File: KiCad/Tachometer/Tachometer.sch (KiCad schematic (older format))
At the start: 24 parts, among them J1 PJ301M-12, Q1 2N3904, Q2 2N3904

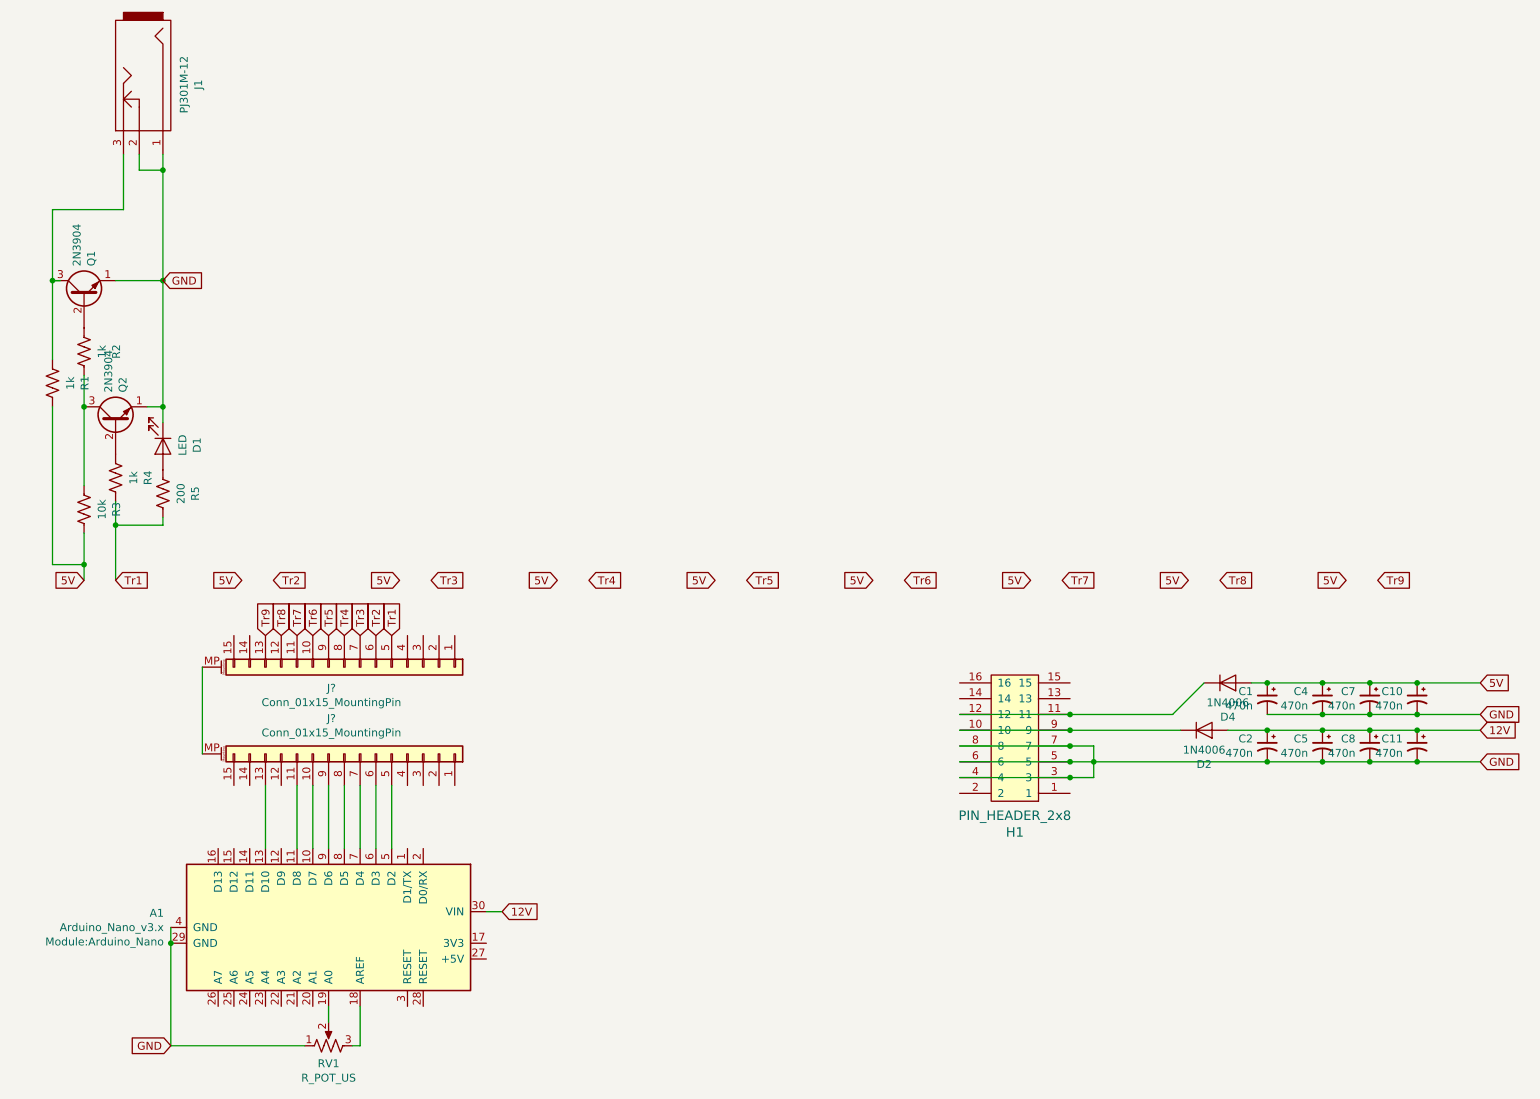
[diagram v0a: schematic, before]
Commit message: ruffplaced pcb
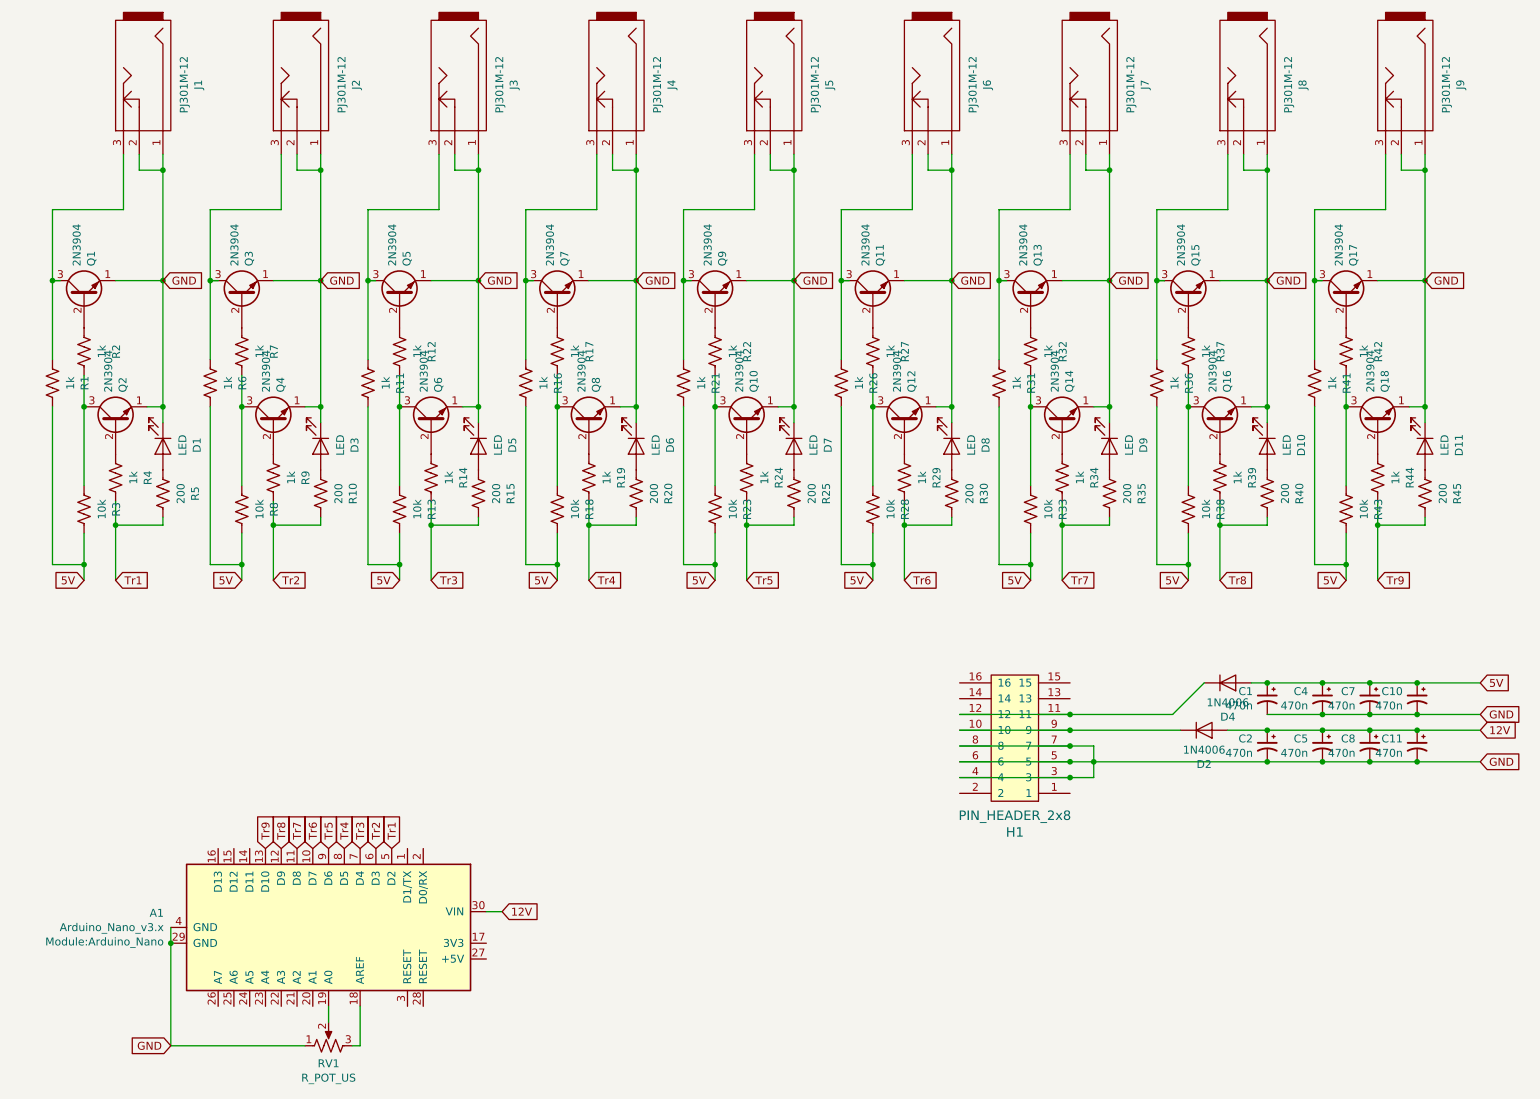
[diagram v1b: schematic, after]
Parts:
- removed J? (x2): Conn_01x15_MountingPin, symbol Connector_Generic_MountingPin:Conn_01x15_MountingPin
- added D10, D11, D3, D5, D6, D7, D8, D9: LED, LED_THT:LED_D3.0mm_FlatTop, symbol Device:LED
- added J2, J3, J4, J5, J6, J7, J8, J9: PJ301M-12, eurorack:PJ301M-12, symbol Eurorack:PJ301M-12
- added Q10, Q11, Q12, Q13, Q14, Q15, Q16, Q17, Q18, Q3, Q4, Q5, Q6, Q7, Q8, Q9: 2N3904, digikey-footprints:SOT-23-3, symbol Transistor_BJT:2N3904
- added R10, R15, R20, R25, R30, R35, R40, R45: 200, Resistor_SMD:R_1206_3216Metric_Pad1.42x1.75mm_HandSolder, symbol Device:R_US
- added R11, R12, R14, R16, R17, R19, R21, R22, R24, R26, R27, R29, R31, R32, R34, R36, R37, R39, R41, R42, R44, R6, R7, R9: 1k, Resistor_SMD:R_1206_3216Metric_Pad1.42x1.75mm_HandSolder, symbol Device:R_US
- added R13, R18, R23, R28, R33, R38, R43, R8: 10k, Resistor_SMD:R_1206_3216Metric_Pad1.42x1.75mm_HandSolder, symbol Device:R_US
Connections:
- wire segments 71 -> 246
